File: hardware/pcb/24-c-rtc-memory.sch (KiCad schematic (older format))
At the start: 10 parts, among them U701 24LC512, U702 DS1307+, Y701 32.768kHz

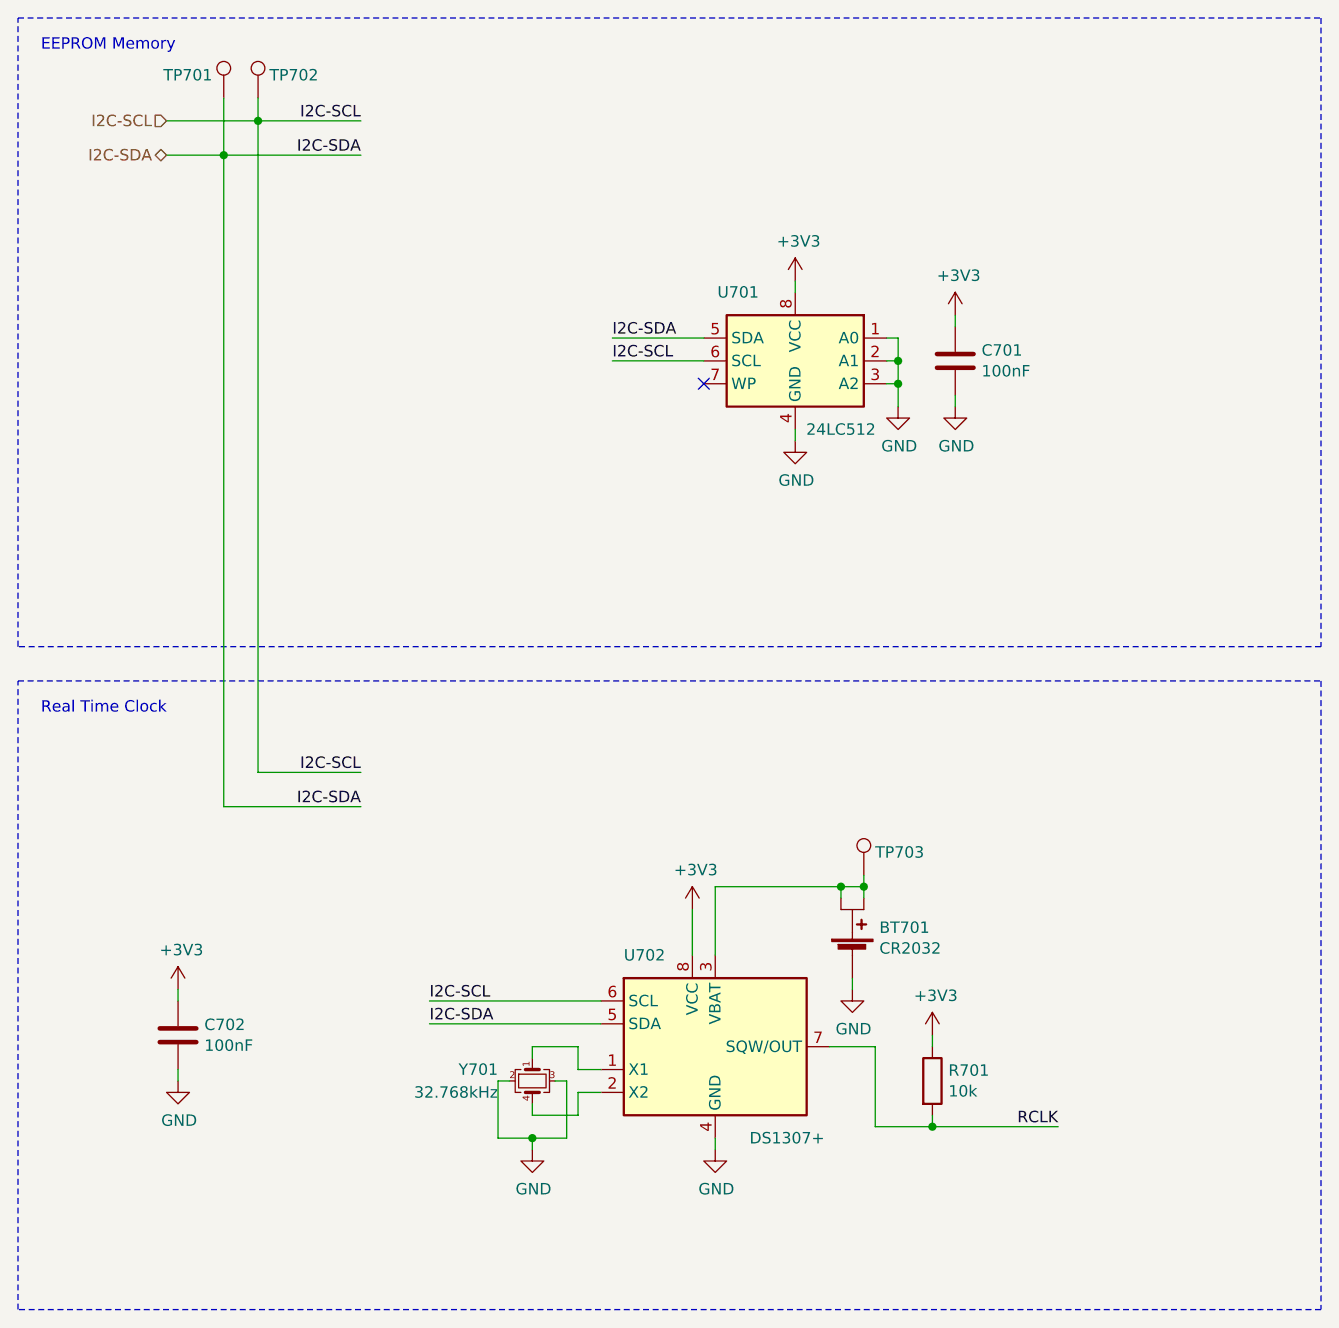
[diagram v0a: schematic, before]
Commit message: Finished PCB (#3)
* Created PCB outline and first placement

* Changed connectors

* Minor

* Included all 3D files

* Mixed changes

* Changed supply to 7V

* Archived PCB project

* Update 24-clocks-rescue.lib

* First placement

* Routed supplies

* Update 24-clocks.kicad_pcb

* Added routing

* Routed more nets

* Finished routing

* Archived project

* Replace hash and date

* minor

* Update pcb.yml

* Update pcb.yml

* Update pcb.yml

* Update pcb.yml

* Auto update commit date and hash

* Update output

* changed outputs

* Added layer to output

* Update hash and date also in sch

* Added caps to hall sensors

* Cleanup files
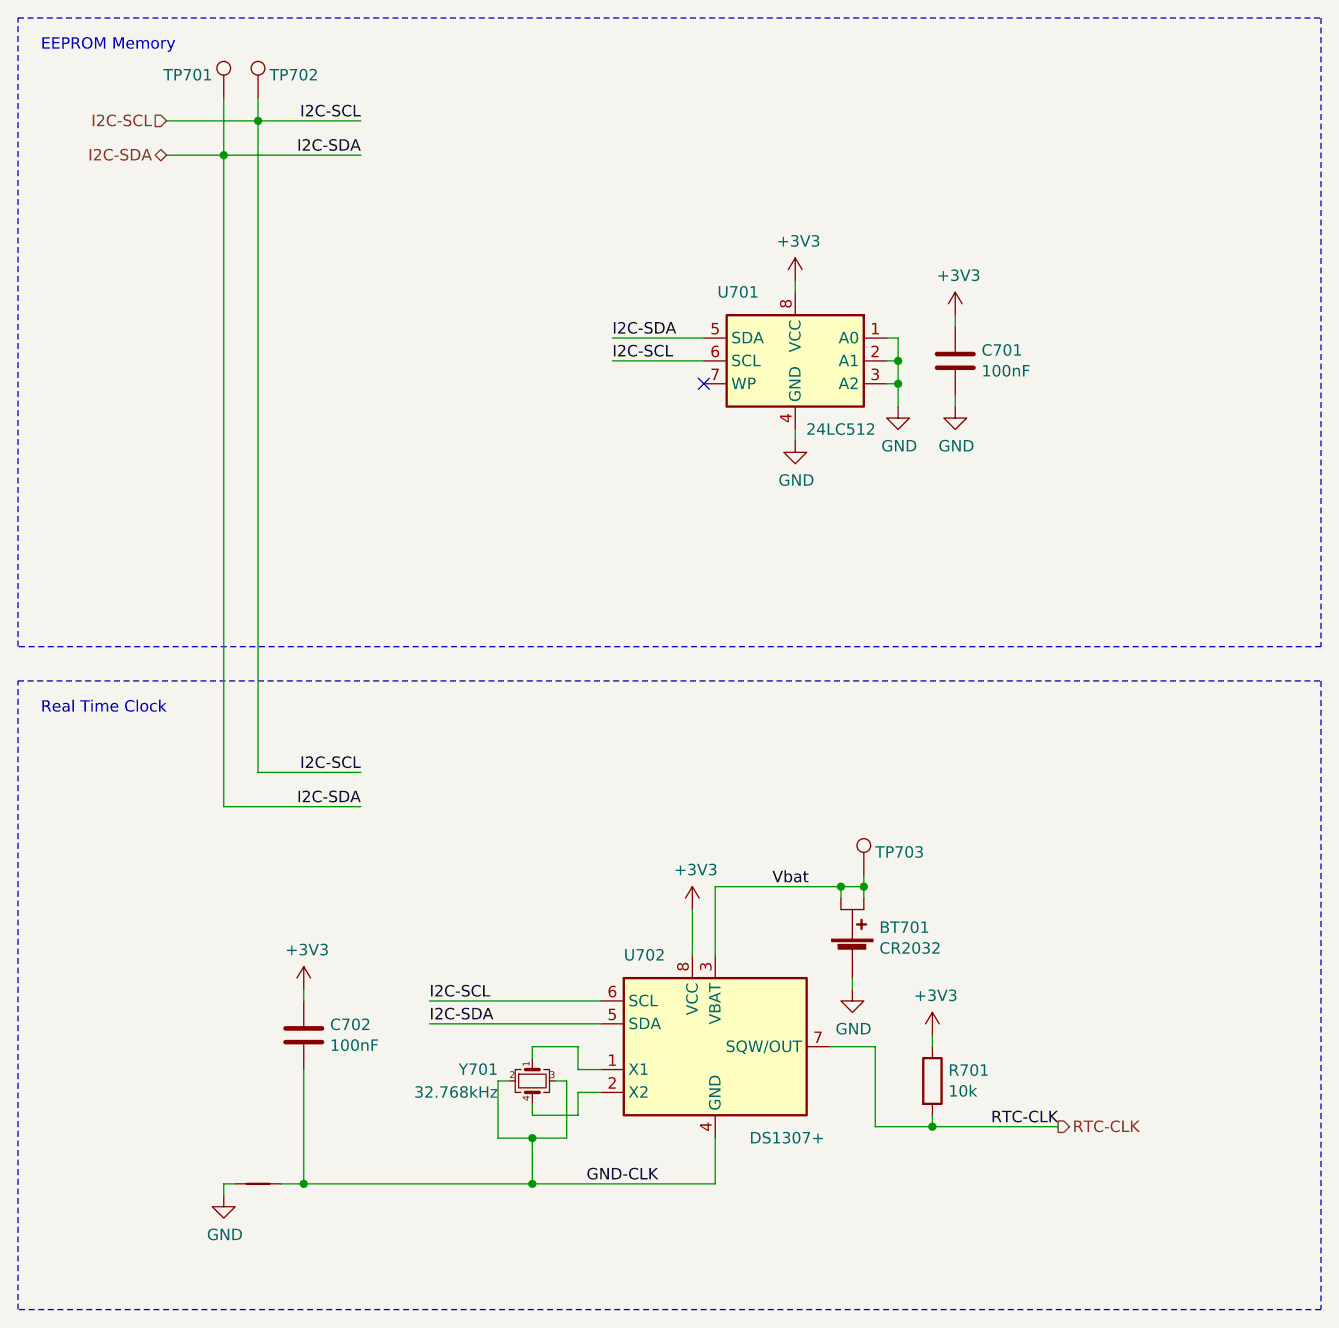
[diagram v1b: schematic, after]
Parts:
- added NT701: Net-Tie_2, NetTie:NetTie-2_SMD_Pad0.5mm, symbol Device:Net-Tie_2
- BT701: Config (none) -> -SLAVE
- U701, U702: footprint Package_SO:SO-8_3.9x4.9mm_P1.27mm -> Package_SO:SOIC-8_3.9x4.9mm_P1.27mm
- Y701: footprint Crystal:Crystal_SMD_SeikoEpson_MC306-4Pin_8.0x3.2mm -> mvl-footprints:Crystal_SMD_SeikoEpson_MC306-4Pin_8.0x3.2mm; Config (none) -> -SLAVE
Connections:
- net GND: now also NT701.2; no longer C702.2, U702.4 (GND), Y701.2, Y701.3
- net Vbat: now reaches BT701.1 (+), BT701.3 (+), TP703.1, U702.3 (VBAT)
- net RCLK renamed RTC-CLK
- new net GND-CLK: C702.2, NT701.1, U702.4 (GND), Y701.2, Y701.3
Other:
- moved on the sheet: C702
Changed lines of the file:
@@
 EESchema Schematic File Version 4
-LIBS:24-clocks-cache
-EELAYER 29 0
+EELAYER 30 0
 EELAYER END
 $Descr A4 11693 8268
@@
 Sheet 7 7
 Title "24 Clocks"
-Date "2020-12-06"
-Rev "V0.x"
+Date "GITDATE"
+Rev "GITHASH"
 Comp "Martin van Leussen"
 Comment1 ""
@@
 F 0 "U701" H 6600 2450 50  0000 C CNN
 F 1 "24LC512" H 6150 1850 50  0000 C CNN
-F 2 "Package_SO:SO-8_3.9x4.9mm_P1.27mm" H 6350 2150 50  0001 C CNN
+F 2 "Package_SO:SOIC-8_3.9x4.9mm_P1.27mm" H 6350 2150 50  0001 C CNN
 F 3 "http://ww1.microchip.com/downloads/en/DeviceDoc/21754M.pdf" H 6350 2150 50  0001 C CNN
 	1    6350 2150
@@
 F 0 "U702" H 5600 5550 50  0000 L CNN
 F 1 "DS1307+" H 6150 4750 50  0000 L CNN
-F 2 "Package_SO:SO-8_3.9x4.9mm_P1.27mm" H 6000 4650 50  0001 C CNN
+F 2 "Package_SO:SOIC-8_3.9x4.9mm_P1.27mm" H 6000 4650 50  0001 C CNN
 F 3 "https://datasheets.maximintegrated.com/en/ds/DS1307.pdf" H 6000 4950 50  0001 C CNN
 F 4 "-SLAVE" H 6000 5150 50  0001 C CNN "Config"
@@
 L power:GND #PWR0711
 U 1 1 5FDCBDE8
-P 6000 5600
-F 0 "#PWR0711" H 6000 5350 50  0001 C CNN
-F 1 "GND" H 6005 5427 50  0000 C CNN
-F 2 "" H 6000 5600 50  0001 C CNN
-F 3 "" H 6000 5600 50  0001 C CNN
-	1    6000 5600
+P 3850 5800
+F 0 "#PWR0711" H 3850 5550 50  0001 C CNN
+F 1 "GND" H 3855 5627 50  0000 C CNN
+F 2 "" H 3850 5800 50  0001 C CNN
+F 3 "" H 3850 5800 50  0001 C CNN
+	1    3850 5800
 	1    0    0    -1
 $EndComp
@@
 	6000 4450 6550 4450
 Wire Wire Line
-	6000 5550 6000 5600
-Wire Wire Line
 	6950 5500 7500 5500
 Connection ~ 6950 5500
 Text Label 7500 5500 2    50   ~ 0
-RCLK
+RTC-CLK
 Wire Wire Line
 	5900 4550 5900 4750
@@
 L Device:C C702
 U 1 1 5FDCBDFD
-P 3650 5100
-F 0 "C702" H 3765 5146 50  0000 L CNN
-F 1 "100nF" H 3765 5055 50  0000 L CNN
-F 2 "Capacitor_SMD:C_0603_1608Metric" H 3688 4950 50  0001 C CNN
-F 3 "~" H 3650 5100 50  0001 C CNN
-F 4 "-SLAVE" H 3650 5100 50  0001 C CNN "Config"
-	1    3650 5100
-	1    0    0    -1
-$EndComp
-$Comp
-L power:GND #PWR0710
-U 1 1 5FDCBE03
-P 3650 5300
-F 0 "#PWR0710" H 3650 5050 50  0001 C CNN
-F 1 "GND" H 3655 5127 50  0000 C CNN
-F 2 "" H 3650 5300 50  0001 C CNN
-F 3 "" H 3650 5300 50  0001 C CNN
-	1    3650 5300
+P 4200 5100
+F 0 "C702" H 4315 5146 50  0000 L CNN
+F 1 "100nF" H 4315 5055 50  0000 L CNN
+F 2 "Capacitor_SMD:C_0603_1608Metric" H 4238 4950 50  0001 C CNN
+F 3 "~" H 4200 5100 50  0001 C CNN
+F 4 "-SLAVE" H 4200 5100 50  0001 C CNN "Config"
+	1    4200 5100
 	1    0    0    -1
 $EndComp
@@
 L power:+3V3 #PWR0707
 U 1 1 5FDCBE09
-P 3650 4900
-F 0 "#PWR0707" H 3650 4750 50  0001 C CNN
-F 1 "+3V3" H 3665 5073 50  0000 C CNN
-F 2 "" H 3650 4900 50  0001 C CNN
-F 3 "" H 3650 4900 50  0001 C CNN
-	1    3650 4900
-	1    0    0    -1
-$EndComp
-Wire Wire Line
-	3650 4900 3650 4950
-Wire Wire Line
-	3650 5250 3650 5300
+P 4200 4900
+F 0 "#PWR0707" H 4200 4750 50  0001 C CNN
+F 1 "+3V3" H 4215 5073 50  0000 C CNN
+F 2 "" H 4200 4900 50  0001 C CNN
+F 3 "" H 4200 4900 50  0001 C CNN
+	1    4200 4900
+	1    0    0    -1
+$EndComp
+Wire Wire Line
+	4200 4900 4200 4950
 Text Label 4450 3950 2    50   ~ 0
 I2C-SCL
@@
 F 0 "Y701" V 5150 5150 50  0000 R CNN
 F 1 "32.768kHz" V 5250 5150 50  0000 R CNN
-F 2 "Crystal:Crystal_SMD_SeikoEpson_MC306-4Pin_8.0x3.2mm" H 5200 5300 50  0001 C CNN
+F 2 "mvl-footprints:Crystal_SMD_SeikoEpson_MC306-4Pin_8.0x3.2mm" H 5200 5300 50  0001 C CNN
 F 3 "~" H 5200 5300 50  0001 C CNN
+F 4 "-SLAVE" H 5200 5300 50  0001 C CNN "Config"
 	1    5200 5300
 	0    1    1    0
@@
 Wire Wire Line
 	5200 5450 5200 5400
-$Comp
-L power:GND #PWR0109
-U 1 1 5FE8D112
-P 5200 5600
-F 0 "#PWR0109" H 5200 5350 50  0001 C CNN
-F 1 "GND" H 5205 5427 50  0000 C CNN
-F 2 "" H 5200 5600 50  0001 C CNN
-F 3 "" H 5200 5600 50  0001 C CNN
-	1    5200 5600
-	1    0    0    -1
-$EndComp
-Wire Wire Line
-	5200 5600 5200 5550
 Wire Wire Line
 	5200 5550 5350 5550
@@
 F 2 "mvl-footprints:BATT_WE_79523141" V 6600 4810 50  0001 C CNN
 F 3 "~" V 6600 4810 50  0001 C CNN
+F 4 "-SLAVE" H 6600 4750 50  0001 C CNN "Config"
 	1    6600 4750
 	1    0    0    -1
@@
 Wire Wire Line
 	6600 4900 6600 4850
+Text Label 6250 4450 0    50   ~ 0
+Vbat
+Text HLabel 7500 5500 2    50   Output ~ 0
+RTC-CLK
+$Comp
+L Device:Net-Tie_2 NT701
+U 1 1 601FC6FC
+P 4000 5750
+F 0 "NT701" V 3954 5794 50  0001 L CNN
+F 1 "Net-Tie_2" V 4045 5794 50  0001 L CNN
+F 2 "NetTie:NetTie-2_SMD_Pad0.5mm" H 4000 5750 50  0001 C CNN
+F 3 "~" H 4000 5750 50  0001 C CNN
+	1    4000 5750
+	-1   0    0    1
+$EndComp
+Text Label 5750 5750 2    50   ~ 0
+GND-CLK
+Wire Wire Line
+	3850 5800 3850 5750
+Wire Wire Line
+	3850 5750 3900 5750
+Wire Wire Line
+	6000 5550 6000 5750
+Wire Wire Line
+	5200 5550 5200 5750
+Connection ~ 5200 5750
+Wire Wire Line
+	5200 5750 6000 5750
+Wire Wire Line
+	4200 5750 5200 5750
+Wire Wire Line
+	4200 5250 4200 5750
+Wire Wire Line
+	4100 5750 4200 5750
+Connection ~ 4200 5750
 $EndSCHEMATC
